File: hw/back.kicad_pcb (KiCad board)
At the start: 2 copper layers, 110 x 55 mm, 77 parts, among them J1 IDC_02X13, J2 FC681495, J3 N42GK-04, Q1 BSC080N03MS, U1 OSRB38C9BA, U2 MCP1826S, U3 MCP1826S, U4 BQ24192, U5 LTC1871, U6 LTC2941CMS8E

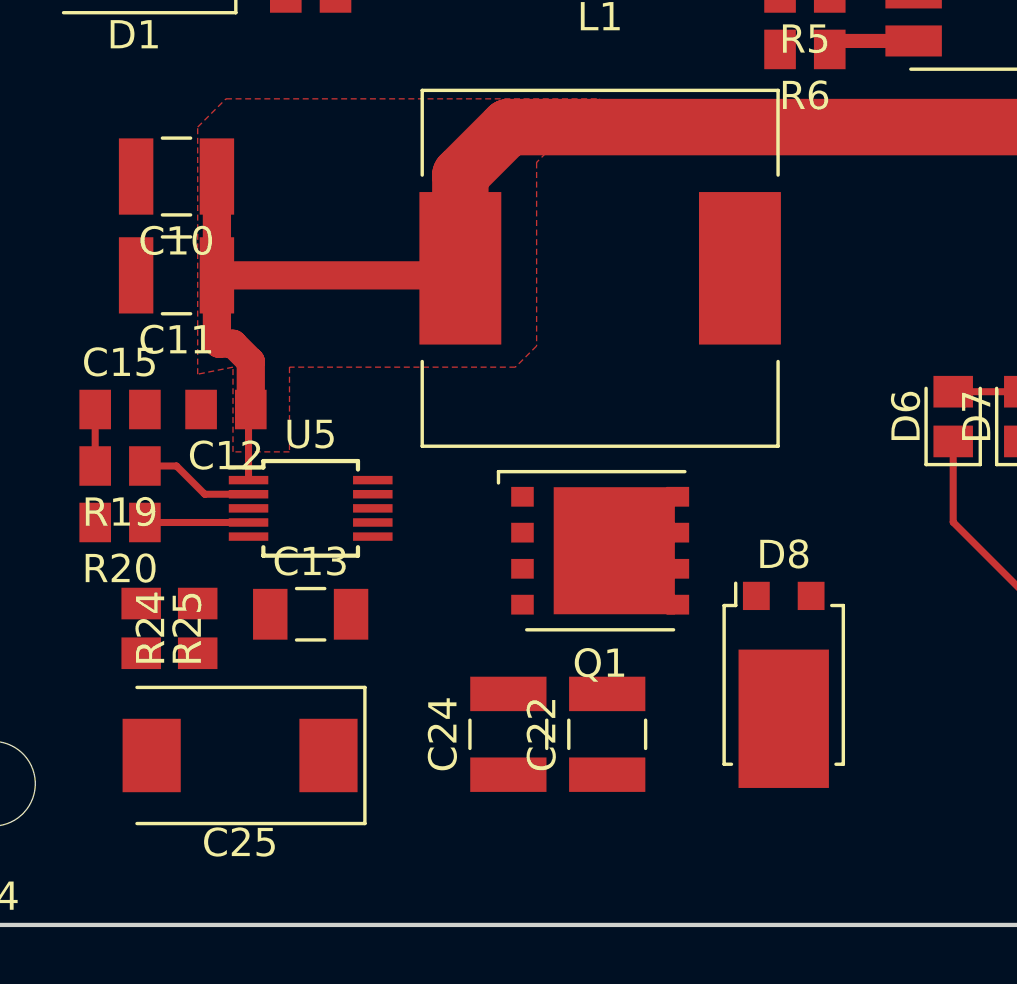
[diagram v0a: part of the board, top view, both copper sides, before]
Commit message: updated pcb
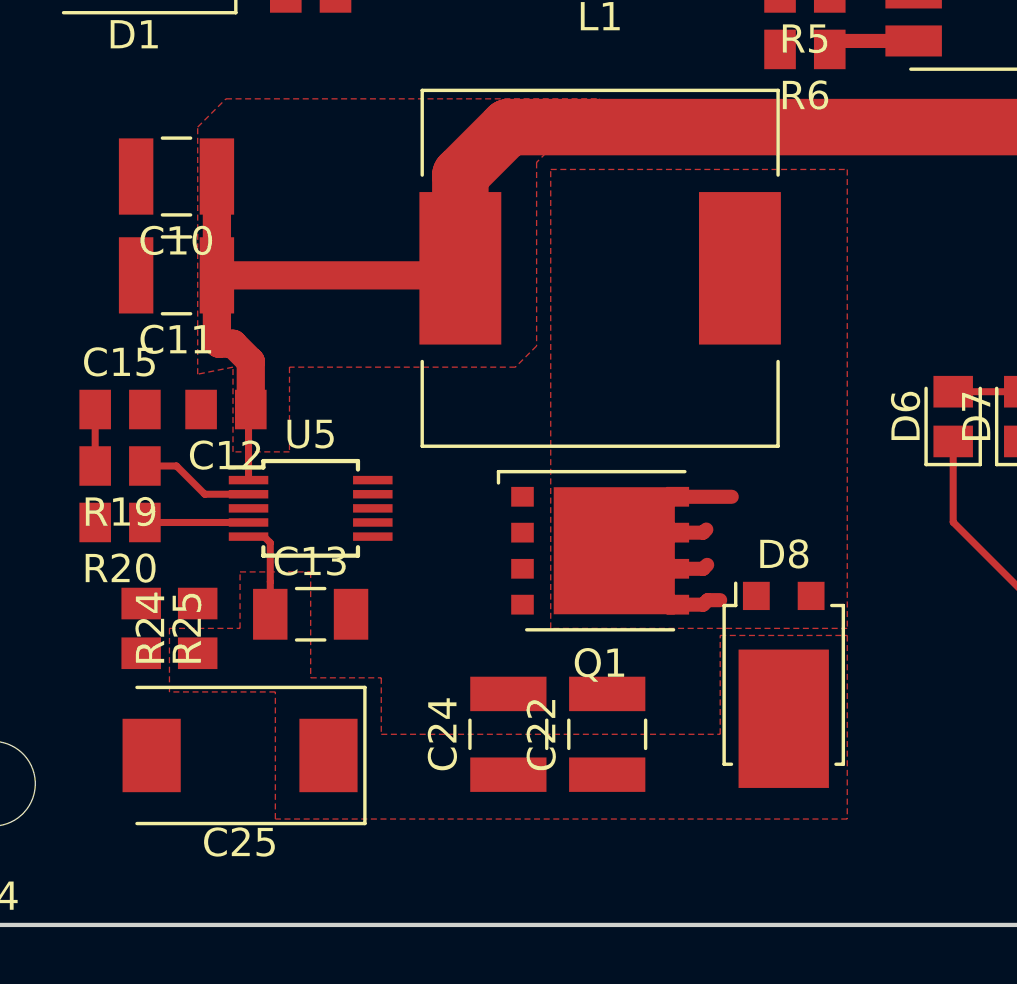
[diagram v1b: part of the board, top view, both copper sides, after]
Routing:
- net Net-(D8-Pad1): track 0.00 -> 11.2 mm
- net +5V5: track 20.3 -> 23.7 mm
- added copper zone on F.Cu, net +5V5
- added copper zone on F.Cu, net Net-(D8-Pad1)
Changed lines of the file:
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@@
     (thickness 1.6)
     (drawings 6)
-    (tracks 323)
+    (tracks 339)
     (zones 0)
     (modules 77)
@@
   )
   (setup
-    (last_trace_width 1)
+    (last_trace_width 0.25)
     (user_trace_width 0.5)
     (user_trace_width 0.8)
@@
   (segment (start 161.525 132.16) (end 161.34 131.975) (width 0.25) (layer F.Cu) (net 2))
   (segment (start 161.34 131.975) (end 159.335 131.975) (width 0.25) (layer F.Cu) (net 2))
+  (segment (start 104.05 126.25) (end 104.6 126.25) (width 0.25) (layer F.Cu) (net 3))
+  (segment (start 104.6 126.25) (end 104.82 126.47) (width 0.25) (layer F.Cu) (net 3))
+  (segment (start 104.82 126.47) (end 104.82 127.85) (width 0.25) (layer F.Cu) (net 3))
+  (segment (start 104.82 127.85) (end 104.82 129) (width 0.25) (layer F.Cu) (net 3))
   (segment (start 141.15 131.15) (end 141.15 129.95) (width 0.25) (layer F.Cu) (net 5))
   (segment (start 141.15 129.95) (end 141.9 129.2) (width 0.25) (layer F.Cu) (net 5))
@@
   (segment (start 165.07 105.3) (end 165.37 105) (width 0.5) (layer F.Cu) (net 47))
   (segment (start 162.4 107) (end 165.37 107) (width 0.5) (layer F.Cu) (net 48))
+  (segment (start 119.25 127.39) (end 120.15 127.39) (width 0.5) (layer F.Cu) (net 49))
+  (segment (start 120.15 127.39) (end 120.29 127.25) (width 0.5) (layer F.Cu) (net 49))
+  (segment (start 120.31 128.5) (end 120.75 128.5) (width 0.5) (layer F.Cu) (net 49))
+  (segment (start 119.25 128.66) (end 120.15 128.66) (width 0.5) (layer F.Cu) (net 49))
+  (segment (start 120.15 128.66) (end 120.31 128.5) (width 0.5) (layer F.Cu) (net 49))
+  (segment (start 119.25 128.66) (end 118.91 128.66) (width 0.5) (layer F.Cu) (net 49))
+  (segment (start 118.91 128.66) (end 117 126.75) (width 0.5) (layer F.Cu) (net 49))
+  (segment (start 119.25 127.39) (end 117.64 127.39) (width 0.5) (layer F.Cu) (net 49))
+  (segment (start 117.64 127.39) (end 117 126.75) (width 0.5) (layer F.Cu) (net 49))
+  (segment (start 119.25 126.11) (end 120.15 126.11) (width 0.5) (layer F.Cu) (net 49))
+  (segment (start 120.15 126.11) (end 120.26 126) (width 0.5) (layer F.Cu) (net 49))
+  (segment (start 119.25 124.84) (end 121.16 124.84) (width 0.5) (layer F.Cu) (net 49))
   (zone (net 5) (net_name GND) (layer F.Cu) (hatch edge 0.508)
     (connect_pads (clearance 0.508))
@@
       )
     )
+  )
+  (zone (net 49) (net_name "Net-(D8-Pad1)") (layer F.Cu) (hatch edge 0.508)
+    (priority 2)
+    (connect_pads (clearance 0.508))
+    (min_thickness 0.254)
+    (fill yes (arc_segments 16) (thermal_gap 0.508) (thermal_bridge_width 0.508))
+    (polygon
+      (pts
+        (xy 114.75 113.25) (xy 125.25 113.25) (xy 125.25 129.5) (xy 114.75 129.5)
+      )
+    )
+  )
+  (zone (net 3) (net_name +5V5) (layer F.Cu) (hatch edge 0.508)
+    (priority 3)
+    (connect_pads (clearance 0.508))
+    (min_thickness 0.254)
+    (fill yes (arc_segments 16) (thermal_gap 0.508) (thermal_bridge_width 0.508))
+    (polygon
+      (pts
+        (xy 120.75 133.25) (xy 120.75 129.75) (xy 125.25 129.75) (xy 125.25 136.25) (xy 105 136.25)
+        (xy 105 131.75) (xy 101.25 131.75) (xy 101.25 129.5) (xy 103.75 129.5) (xy 103.75 127.5)
+        (xy 106.25 127.5) (xy 106.25 131.25) (xy 108.75 131.25) (xy 108.75 133.25)
+      )
+    )
